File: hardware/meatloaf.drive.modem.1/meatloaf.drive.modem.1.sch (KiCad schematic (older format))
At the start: 13 parts, among them J1 IEC SERIAL PORT, J2 User Port, SW1 PREVIOUS, SW2 SELECT, SW3 NEXT, SW4 MODE / RESET, U1 ESP-12F

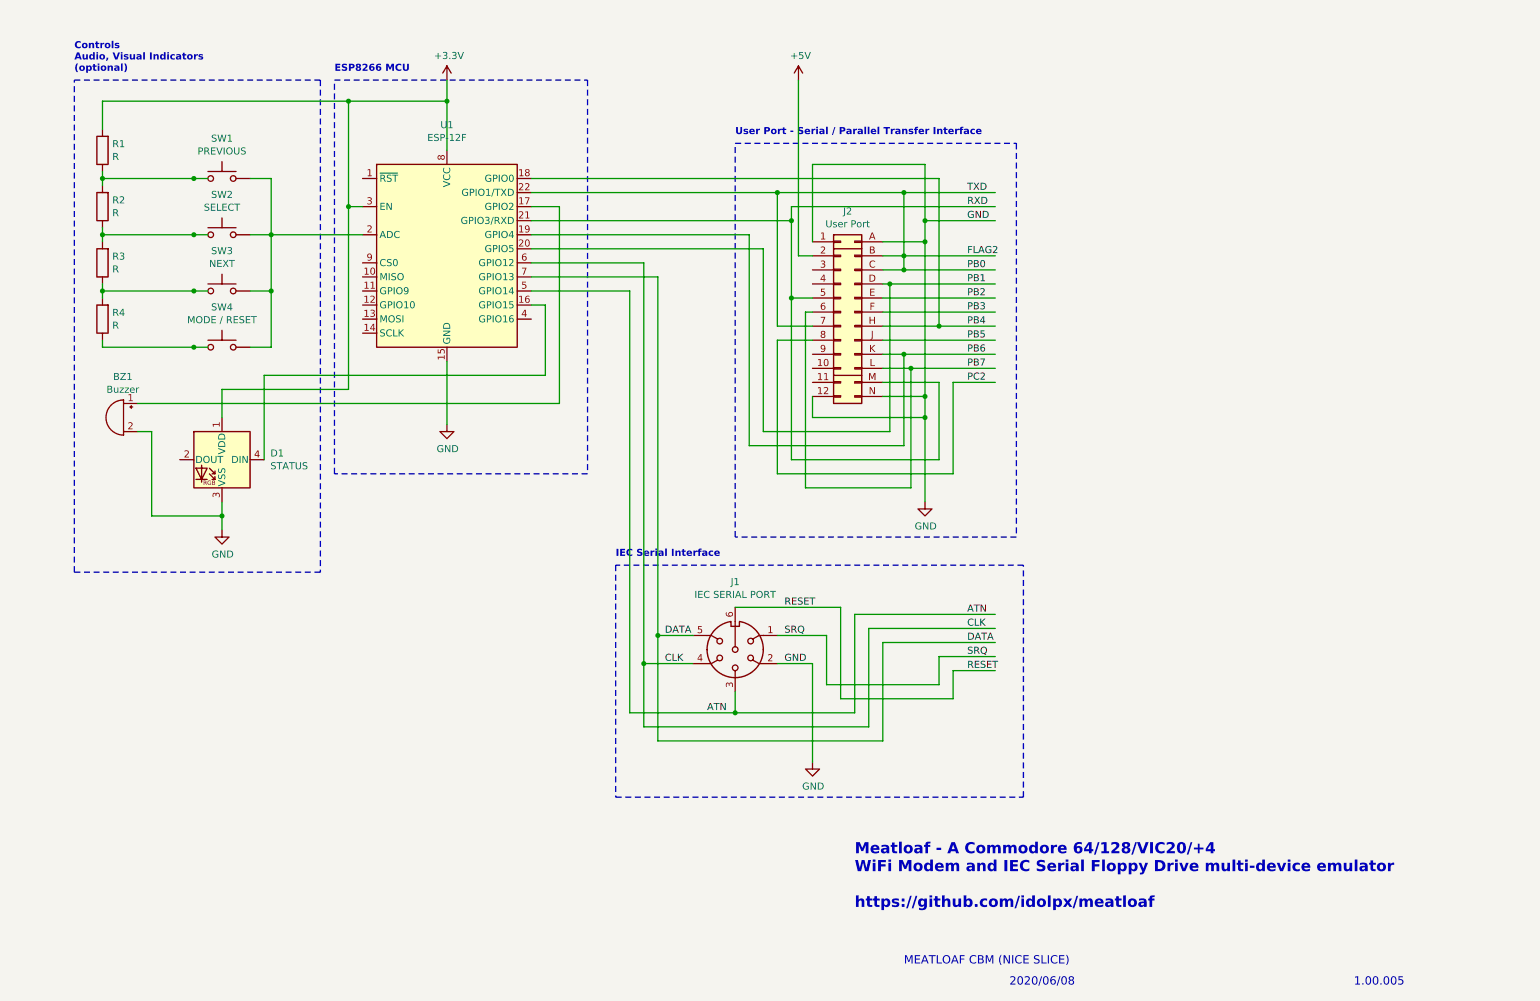
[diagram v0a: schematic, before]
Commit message: more debug
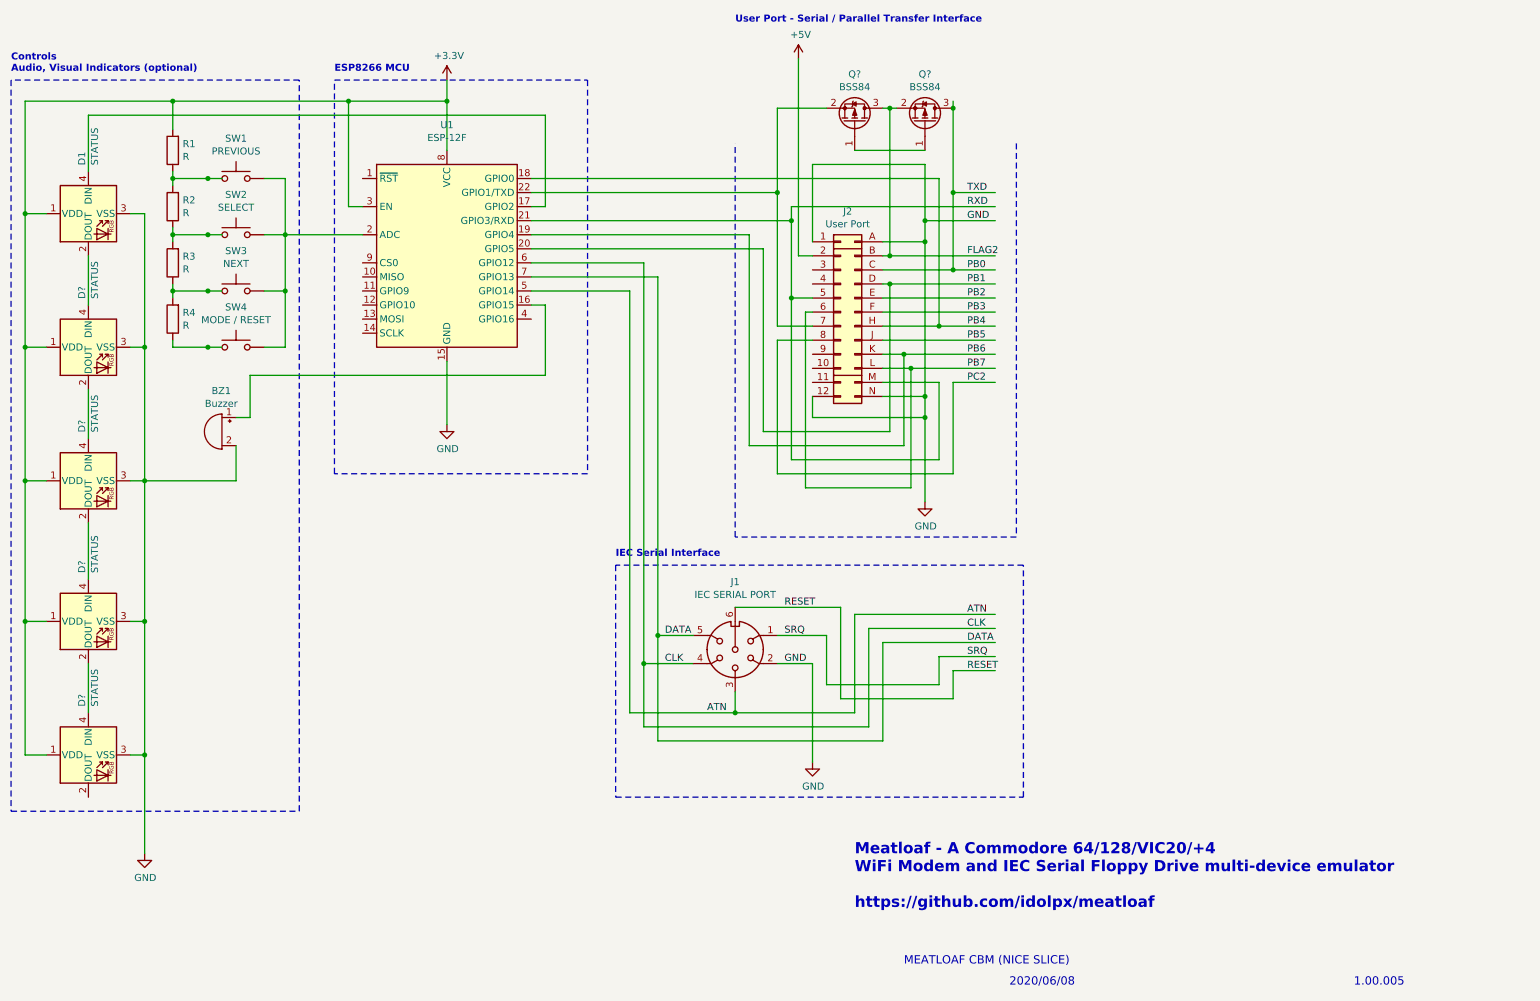
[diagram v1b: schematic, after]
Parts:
- added D? (x4): STATUS, LED_SMD:LED_WS2812B_PLCC4_5.0x5.0mm_P3.2mm, symbol LED:WS2812B
- added Q? (x2): BSS84, Package_TO_SOT_SMD:SOT-23, symbol Transistor_FET:BSS84
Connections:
- wire segments 143 -> 170
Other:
- note added: "Controls\nAudio, Visual Indicators (optional)"
- note removed: "Controls\nAudio, Visual Indicators\n(optional)"
- moved on the sheet: BZ1, D1, R1, R2, R3, R4, SW1, SW2, SW3, SW4
